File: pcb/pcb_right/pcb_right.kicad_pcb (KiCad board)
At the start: 2 copper layers, 154 x 108.3 mm, 61 parts, among them U1 Nice_Nano_V2

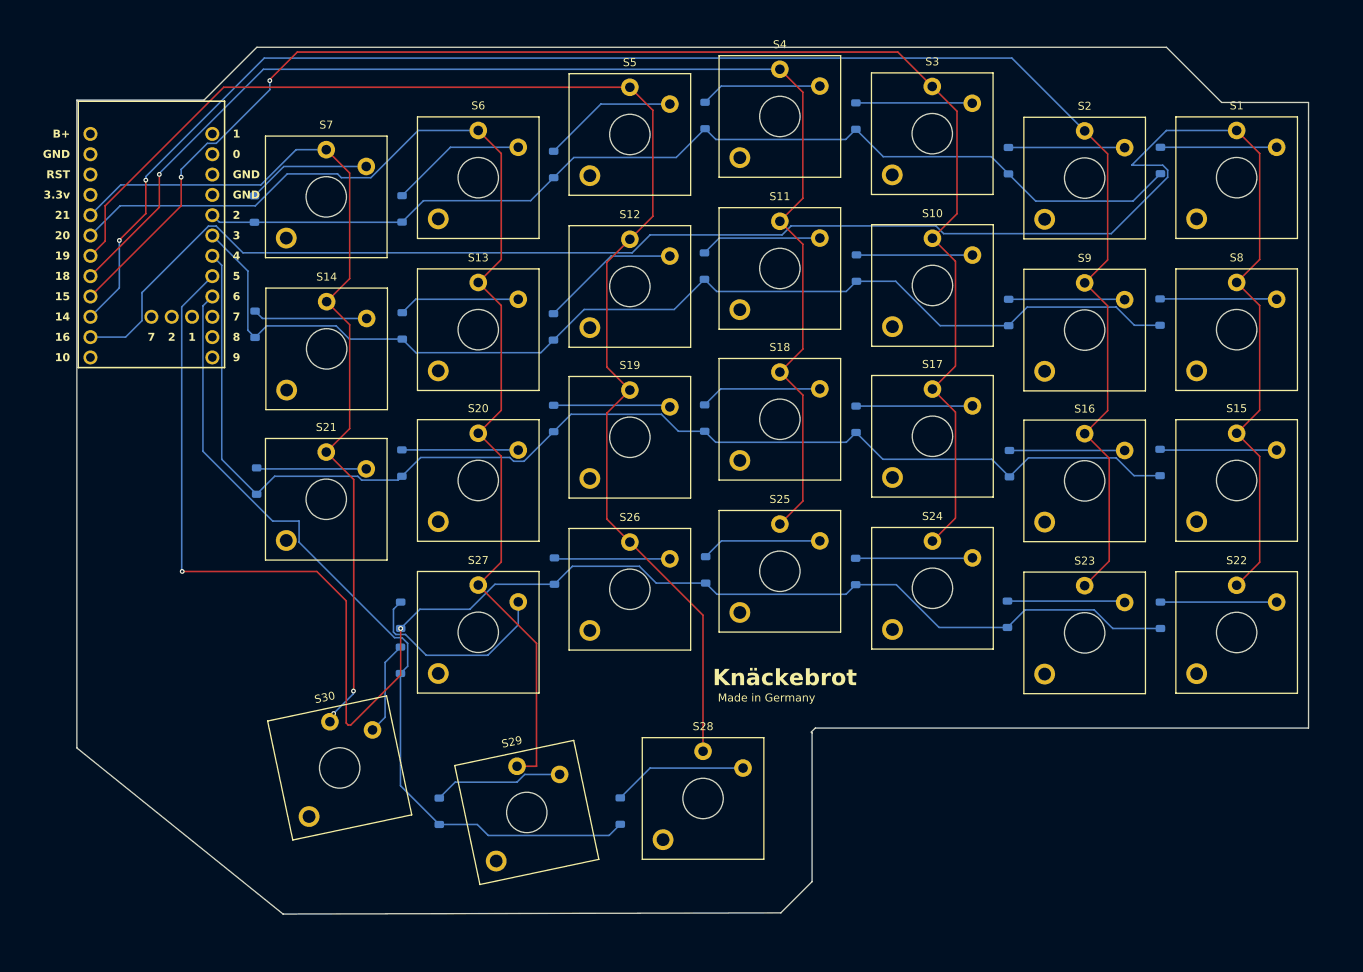
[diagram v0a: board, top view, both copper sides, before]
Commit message: Upadate v1.00
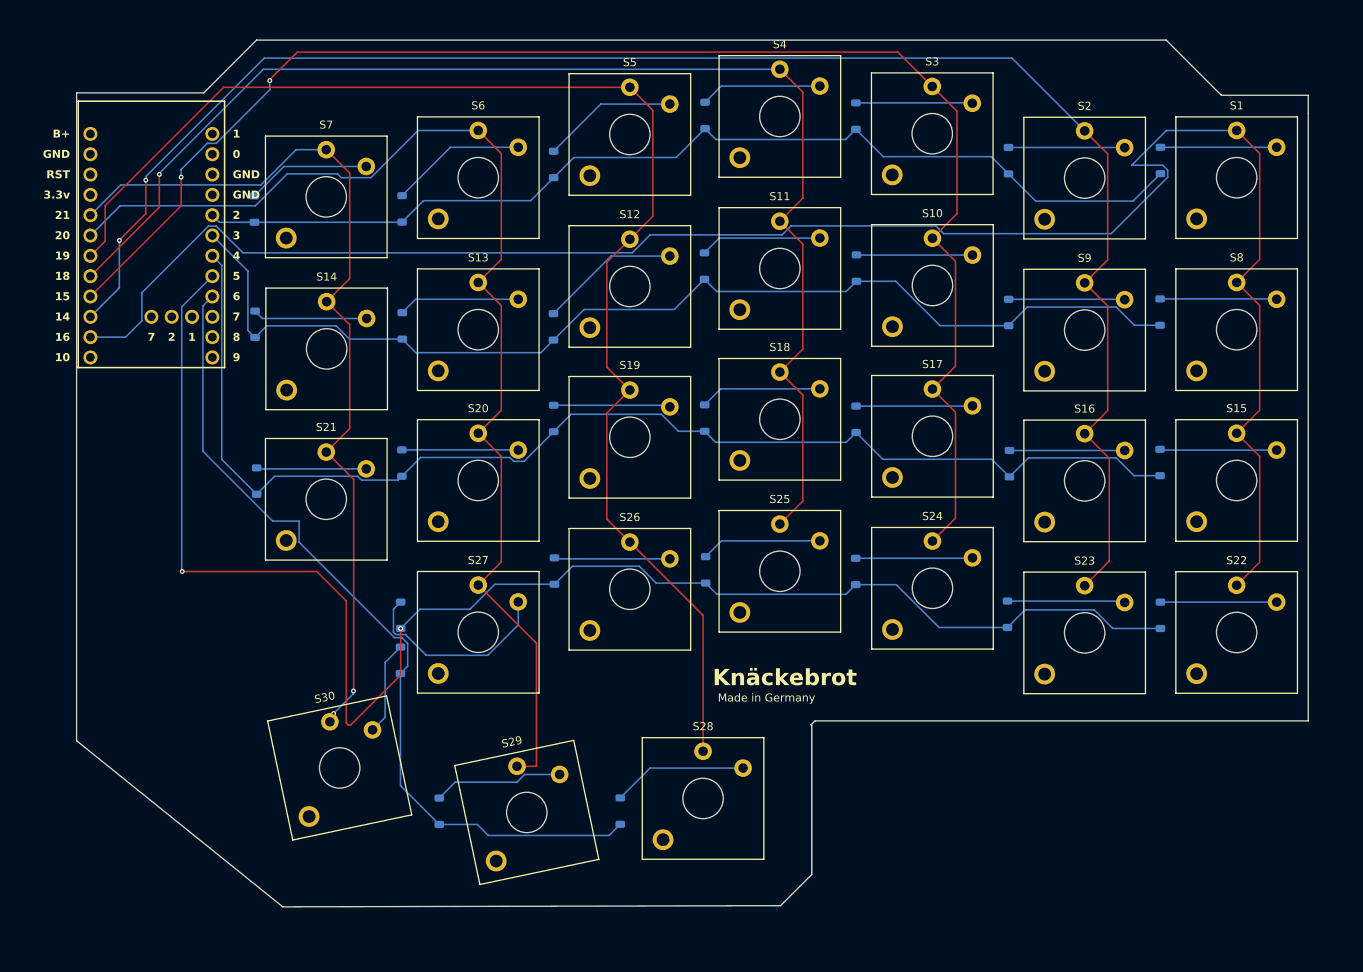
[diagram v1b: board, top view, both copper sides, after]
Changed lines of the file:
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@@
 	(gr_poly
 		(pts
-			(xy 215.442618 46.16) (xy 215.442618 43.9) (xy 204.582618 43.9) (xy 197.682618 37) (xy 83.982618 37)
-			(xy 77.382618 43.6) (xy 61.482618 43.6) (xy 61.482618 124.583333) (xy 87.254951 145.344379) (xy 149.482618 145.2)
-			(xy 153.382618 141.3) (xy 153.382618 122.7) (xy 153.282618 122.6) (xy 153.782618 122.1) (xy 215.442618 122.1)
-			(xy 215.442618 46.16)
+			(xy 215.41 45.26) (xy 215.41 43) (xy 204.55 43) (xy 197.65 36.1) (xy 83.95 36.1) (xy 77.35 42.7)
+			(xy 61.45 42.7) (xy 61.45 123.683333) (xy 87.222333 144.444379) (xy 149.45 144.3) (xy 153.35 140.4)
+			(xy 153.35 121.8) (xy 153.25 121.7) (xy 153.75 121.2) (xy 215.41 121.2) (xy 215.41 45.26)
 		)
 		(stroke

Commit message: Upadate v1.00
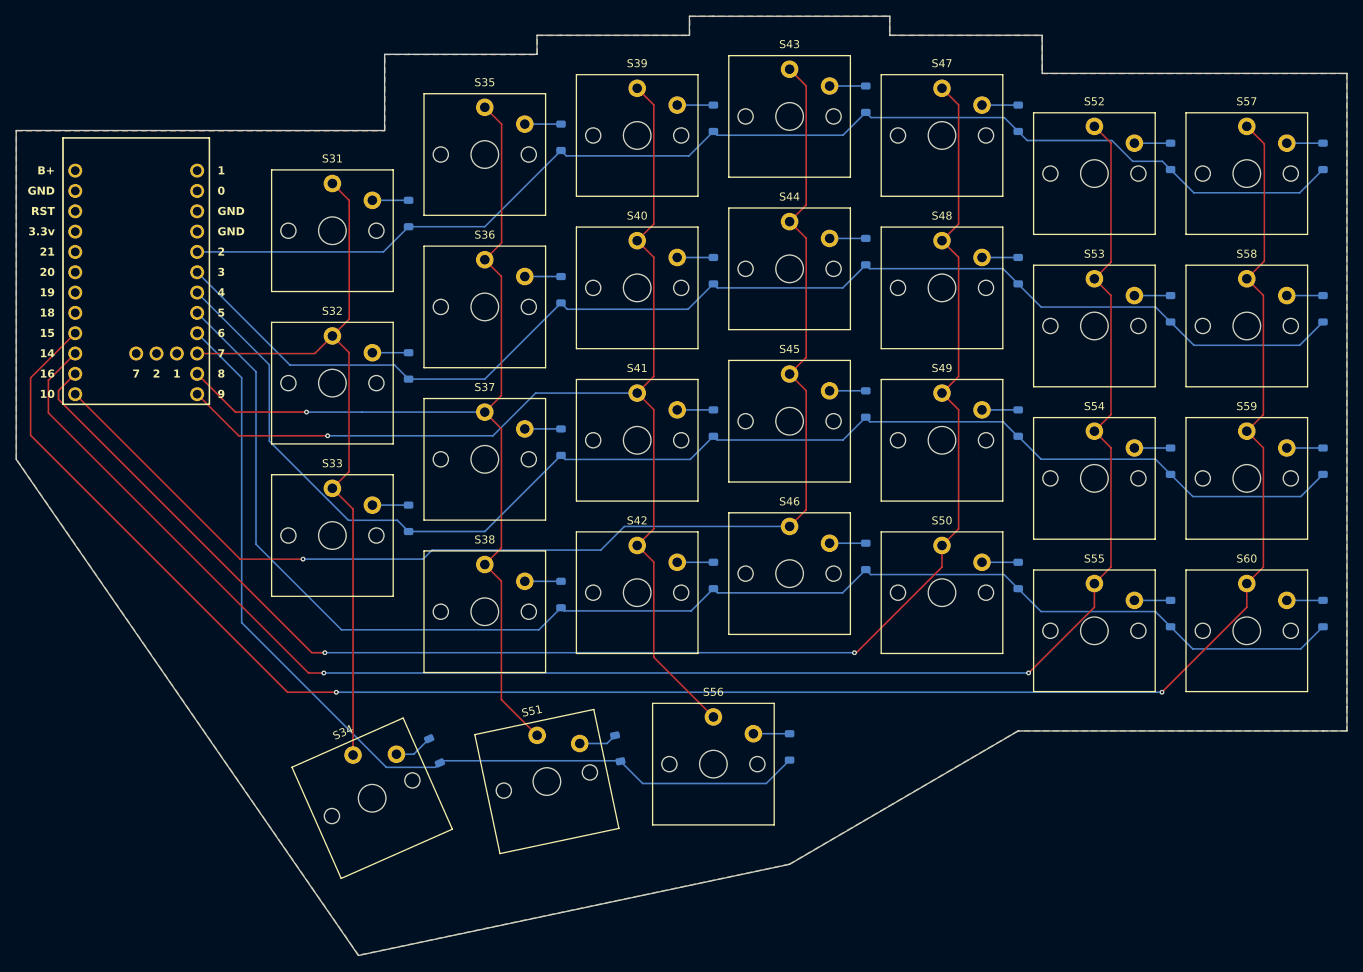
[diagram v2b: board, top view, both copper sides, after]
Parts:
- removed D1, D10, D11, D12, D13, D14, D15, D16, D17, D18, D19, D2, D20, D21, D22, D23, D24, D25, D26, D27, D28, D29, D3, D30, D4, D5, D6, D7, D8, D9: Diode, Diode_SMD:D_SOD-123
- removed S1, S10, S11, S12, S13, S14, S15, S16, S17, S18, S19, S2, S20, S21, S22, S23, S24, S25, S26, S27, S28, S29, S3, S30, S4, S5, S6, S7, S8, S9: Keyswitch, ScottoKeebs_Choc:Choc_V2
- removed U1: Nice_Nano_V2, ScottoKeebs_MCU:Nice_Nano_V2
- added D31: Diode, ScottoKeebs_Components:Diode_SOD-123, B.Cu at (103.0, 57.8)
- added D32: Diode, ScottoKeebs_Components:Diode_SOD-123, B.Cu at (103.0, 76.8)
- added D33: Diode, ScottoKeebs_Components:Diode_SOD-123, B.Cu at (103.0, 95.9)
- added D34: Diode, ScottoKeebs_Components:Diode_SOD-123, B.Cu at (106.2, 124.9)
- added D35: Diode, ScottoKeebs_Components:Diode_SOD-123, B.Cu at (122.0, 48.3)
- added D36: Diode, ScottoKeebs_Components:Diode_SOD-123, B.Cu at (122.0, 67.3)
- added D37: Diode, ScottoKeebs_Components:Diode_SOD-123, B.Cu at (122.0, 86.4)
- added D38: Diode, ScottoKeebs_Components:Diode_SOD-123, B.Cu at (122.0, 105.4)
- added D39: Diode, ScottoKeebs_Components:Diode_SOD-123, B.Cu at (141.1, 45.9)
- added D40: Diode, ScottoKeebs_Components:Diode_SOD-123, B.Cu at (141.1, 64.9)
- added D41: Diode, ScottoKeebs_Components:Diode_SOD-123, B.Cu at (141.1, 84.0)
- added D42: Diode, ScottoKeebs_Components:Diode_SOD-123, B.Cu at (141.1, 103.0)
- added D43: Diode, ScottoKeebs_Components:Diode_SOD-123, B.Cu at (160.1, 43.5)
- added D44: Diode, ScottoKeebs_Components:Diode_SOD-123, B.Cu at (160.1, 62.5)
- added D45: Diode, ScottoKeebs_Components:Diode_SOD-123, B.Cu at (160.1, 81.6)
- added D46: Diode, ScottoKeebs_Components:Diode_SOD-123, B.Cu at (160.1, 100.6)
- added D47: Diode, ScottoKeebs_Components:Diode_SOD-123, B.Cu at (179.2, 45.9)
- added D48: Diode, ScottoKeebs_Components:Diode_SOD-123, B.Cu at (179.1, 64.9)
- added D49: Diode, ScottoKeebs_Components:Diode_SOD-123, B.Cu at (179.2, 84.0)
- added D50: Diode, ScottoKeebs_Components:Diode_SOD-123, B.Cu at (179.2, 103.0)
- added D51: Diode, ScottoKeebs_Components:Diode_SOD-123, B.Cu at (129.1, 124.6)
- added D52: Diode, ScottoKeebs_Components:Diode_SOD-123, B.Cu at (198.2, 50.6)
- added D53: Diode, ScottoKeebs_Components:Diode_SOD-123, B.Cu at (198.2, 69.7)
- added D54: Diode, ScottoKeebs_Components:Diode_SOD-123, B.Cu at (198.2, 88.7)
- added D55: Diode, ScottoKeebs_Components:Diode_SOD-123, B.Cu at (198.2, 107.8)
- added D56: Diode, ScottoKeebs_Components:Diode_SOD-123, B.Cu at (150.6, 124.5)
- added D57: Diode, ScottoKeebs_Components:Diode_SOD-123, B.Cu at (217.2, 50.6)
- added D58: Diode, ScottoKeebs_Components:Diode_SOD-123, B.Cu at (217.2, 69.7)
- added D59: Diode, ScottoKeebs_Components:Diode_SOD-123, B.Cu at (217.2, 88.7)
- added D60: Diode, ScottoKeebs_Components:Diode_SOD-123, B.Cu at (217.3, 107.8)
- added S31: Keyswitch, ScottoKeebs_Choc:Choc_V1, F.Cu at (93.4, 59.9)
- added S32: Keyswitch, ScottoKeebs_Choc:Choc_V1, F.Cu at (93.4, 79.0)
- added S33: Keyswitch, ScottoKeebs_Choc:Choc_V1, F.Cu at (93.4, 98.0)
- added S34: Keyswitch, ScottoKeebs_Choc:Choc_V1, F.Cu at (98.4, 130.9)
- added S35: Keyswitch, ScottoKeebs_Choc:Choc_V1, F.Cu at (112.5, 50.4)
- added S36: Keyswitch, ScottoKeebs_Choc:Choc_V1, F.Cu at (112.5, 69.5)
- added S37: Keyswitch, ScottoKeebs_Choc:Choc_V1, F.Cu at (112.5, 88.5)
- added S38: Keyswitch, ScottoKeebs_Choc:Choc_V1, F.Cu at (112.5, 107.6)
- added S39: Keyswitch, ScottoKeebs_Choc:Choc_V1, F.Cu at (131.5, 48.0)
- added S40: Keyswitch, ScottoKeebs_Choc:Choc_V1, F.Cu at (131.5, 67.1)
- added S41: Keyswitch, ScottoKeebs_Choc:Choc_V1, F.Cu at (131.5, 86.1)
- added S42: Keyswitch, ScottoKeebs_Choc:Choc_V1, F.Cu at (131.5, 105.2)
- added S43: Keyswitch, ScottoKeebs_Choc:Choc_V1, F.Cu at (150.6, 45.6)
- added S44: Keyswitch, ScottoKeebs_Choc:Choc_V1, F.Cu at (150.6, 64.7)
- added S45: Keyswitch, ScottoKeebs_Choc:Choc_V1, F.Cu at (150.6, 83.7)
- added S46: Keyswitch, ScottoKeebs_Choc:Choc_V1, F.Cu at (150.6, 102.8)
- added S47: Keyswitch, ScottoKeebs_Choc:Choc_V1, F.Cu at (169.6, 48.0)
- added S48: Keyswitch, ScottoKeebs_Choc:Choc_V1, F.Cu at (169.6, 67.1)
- added S49: Keyswitch, ScottoKeebs_Choc:Choc_V1, F.Cu at (169.6, 86.1)
- added S50: Keyswitch, ScottoKeebs_Choc:Choc_V1, F.Cu at (169.6, 105.2)
- added S51: Keyswitch, ScottoKeebs_Choc:Choc_V1, F.Cu at (120.2, 128.8)
- added S52: Keyswitch, ScottoKeebs_Choc:Choc_V1, F.Cu at (188.7, 52.8)
- added S53: Keyswitch, ScottoKeebs_Choc:Choc_V1, F.Cu at (188.7, 71.8)
- added S54: Keyswitch, ScottoKeebs_Choc:Choc_V1, F.Cu at (188.7, 90.9)
- added S55: Keyswitch, ScottoKeebs_Choc:Choc_V1, F.Cu at (188.7, 109.9)
- added S56: Keyswitch, ScottoKeebs_Choc:Choc_V1, F.Cu at (141.1, 126.6)
- added S57: Keyswitch, ScottoKeebs_Choc:Choc_V1, F.Cu at (207.7, 52.8)
- added S58: Keyswitch, ScottoKeebs_Choc:Choc_V1, F.Cu at (207.7, 71.8)
- added S59: Keyswitch, ScottoKeebs_Choc:Choc_V1, F.Cu at (207.7, 90.9)
- added S60: Keyswitch, ScottoKeebs_Choc:Choc_V1, F.Cu at (207.7, 109.9)
- added U2: Nice_Nano_V2, ScottoKeebs_MCU:Nice_Nano_V2, B.Cu at (68.9, 66.1)
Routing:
- net column 13: track 0.00 -> 250.2 mm, vias 0 -> 2
- net Col_6: track 233.1 -> 0.00 mm
- net column 12: track 0.00 -> 221.7 mm, vias 0 -> 2
- net Col_5: track 211.8 -> 0.00 mm, vias 2 -> 0
- net column 11: track 0.00 -> 197.1 mm, vias 0 -> 2
- net Row_3: track 195.4 -> 0.00 mm, vias 2 -> 0
- net Col_4: track 187.2 -> 0.00 mm, vias 2 -> 0
- net row 8: track 0.00 -> 178.9 mm
- net Col_2: track 172.7 -> 0.00 mm
- net row 7: track 0.00 -> 170.7 mm
- net Col_3: track 163.4 -> 0.00 mm, vias 1 -> 0
- net column 10: track 0.00 -> 161.8 mm, vias 0 -> 1
- net row 6: track 0.00 -> 158.6 mm
- net Row_2: track 156.1 -> 0.00 mm
- net row 5: track 0.00 -> 154.3 mm
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- added copper zone on B.Cu, net GND
- added copper zone on F.Cu, net GND
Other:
- board size 154 x 108.3 mm -> 166.4 x 117.4 mm
- board text removed: "Knäckebrot"
- board text removed: "Made in Germany"
